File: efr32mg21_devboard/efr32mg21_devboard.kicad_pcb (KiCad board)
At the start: 2 copper layers, 50 x 50 mm, 23 parts, among them CON1 CORTEX-DEBUGGER, J1 Conn_01x10, J2 microusb, J3 Conn_01x10, U1 EFR32MG21A020F768IM32-BR, U2 TLV70033_SOT23-5, Y1 38.4MHz, Y2 32.768k

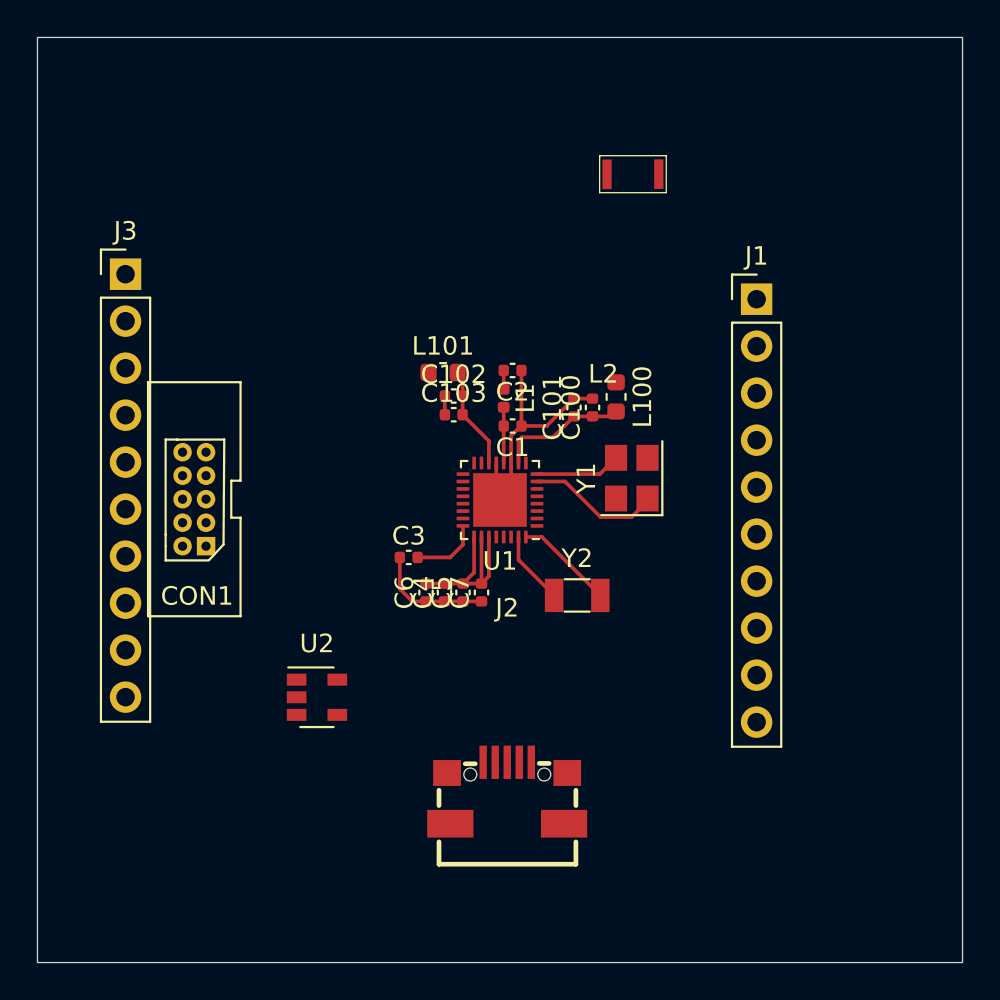
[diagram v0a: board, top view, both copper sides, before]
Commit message: v1.0
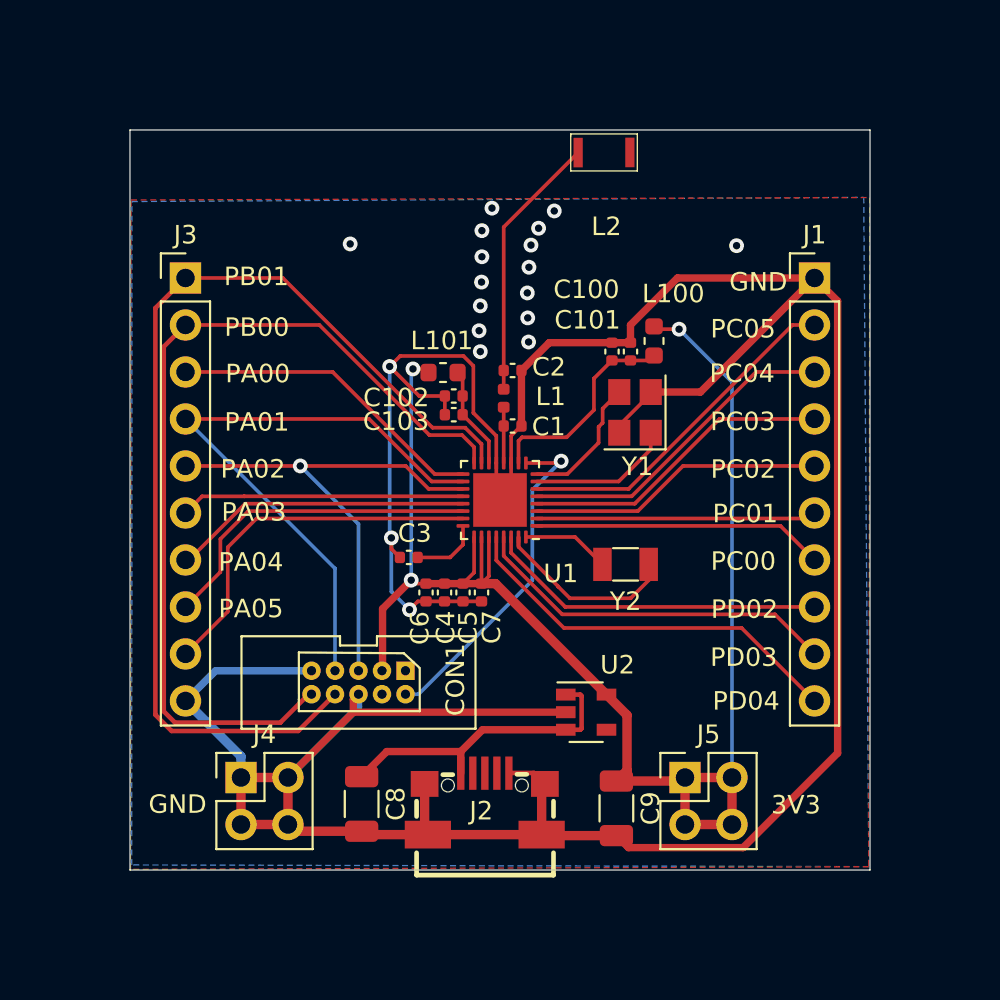
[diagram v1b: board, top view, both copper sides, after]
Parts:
- added C8: C, Capacitor_SMD:C_1206_3216Metric, F.Cu at (142.5, 116.4)
- added C9: C, Capacitor_SMD:C_1206_3216Metric, F.Cu at (156.3, 116.7)
- added J4: Conn_02x02_Counter_Clockwise, Connector_PinHeader_2.54mm:PinHeader_2x02_P2.54mm_Vertical, F.Cu at (136.0, 115.0)
- added J5: Conn_02x02_Counter_Clockwise, Connector_PinHeader_2.54mm:PinHeader_2x02_P2.54mm_Vertical, F.Cu at (160.0, 115.0)
- moved U2 14.6 mm to (154.7, 111.5)
- moved CON1 13.3 mm to (142.4, 109.9), turned to 270 degrees
- moved C100 3.65 mm to (157.1, 92.0)
- moved C101 3.65 mm to (156.1, 92.0)
- moved L100 3.65 mm to (158.3, 91.4)
- moved Y1 3.56 mm to (157.3, 95.3)
- moved J1 3.33 mm to (167.0, 88.0)
- moved J3 3.25 mm to (133.0, 88.0)
- moved Y2 3.10 mm to (156.8, 103.5), turned to 180 degrees
- moved L2 1.95 mm to (154.0, 82.0)
- moved J2 1.35 mm to (149.2, 116.4)
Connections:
- CON1 pad 10: Net-(CON1-Pad10) -> PB00
- CON1 pad 8: Net-(CON1-Pad8) -> PB01
- J1 pad 1: Net-(J1-Pad1) -> GND
- J2 pad 0: Net-(J2-Pad0) -> GND
- J2 pad 1: Net-(J2-Pad1) -> Net-(C8-Pad1)
- J2 pad 5: Net-(J2-Pad5) -> GND
- J3 pad 10: Net-(J3-Pad10) -> GND
- U2 pad 1: Net-(U2-Pad1) -> Net-(C8-Pad1)
- U2 pad 2: Net-(U2-Pad2) -> GND
- U2 pad 3: Net-(U2-Pad3) -> Net-(C8-Pad1)
- U2 pad 5: Net-(U2-Pad5) -> +3V3
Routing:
- net GND: track 21.4 -> 189.7 mm, vias 0 -> 19
- net +3V3: track 11.0 -> 85.2 mm, vias 0 -> 3
- net PB01: track 0.00 -> 55.9 mm
- net PB00: track 0.00 -> 49.4 mm
- net PA01: track 0.00 -> 33.4 mm
- net PA02: track 0.00 -> 27.9 mm, vias 0 -> 1
- net PD04: track 0.00 -> 21.6 mm
- net PA06: track 0.00 -> 20.1 mm
- net PD03: track 0.00 -> 20.0 mm
- net PC05: track 0.00 -> 18.7 mm
- net PD02: track 0.00 -> 18.5 mm
- net RESETn: track 0.00 -> 18.4 mm, vias 0 -> 1
- net PA05: track 0.00 -> 18.2 mm
- net PC04: track 0.00 -> 17.8 mm
- net Net-(C8-Pad1): track 0.00 -> 17.4 mm
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- added copper zone on B.Cu, net (none)
- added copper zone on F.Cu, net GND
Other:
- board size 50 x 50 mm -> 40 x 40 mm
- board text added: "3V3"
- board text added: "GND"
- board text added: "PA00"
- board text added: "PA01"
- board text added: "PA02"
- board text added: "PA03"
- board text added: "PA04"
- board text added: "PA05"
- board text added: "PA06"
- board text added: "PB00"
- board text added: "PB01"
- board text added: "PC00"
- board text added: "PC01"
- board text added: "PC02"
- board text added: "PC03"
- board text added: "PC04"
- board text added: "PC05"
- board text added: "PD02"
- board text added: "PD03"
- board text added: "PD04"
